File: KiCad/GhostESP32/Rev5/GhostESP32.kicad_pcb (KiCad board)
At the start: 2 copper layers, 76.7 x 56.7 mm, 52 parts, among them J1 USB_OTG, J2 CONN_01X12, J3 CONN_01X12, J4 STEERING, J5 MOTOR, Q1 Q_NPN_BEC, Q2 Q_NPN_BEC, Q3 Q_NPN_BEC, Q4 BSS138, Q5 BSS138, SW1 SW_SPDT, U1 NCP1117-3.3_SOT223, U2 CP2102, U3 TMP102, U4 MPU-9250, U5 ESP-WROOM-32, U6 NeoPixelNano, U7 NeoPixelNano

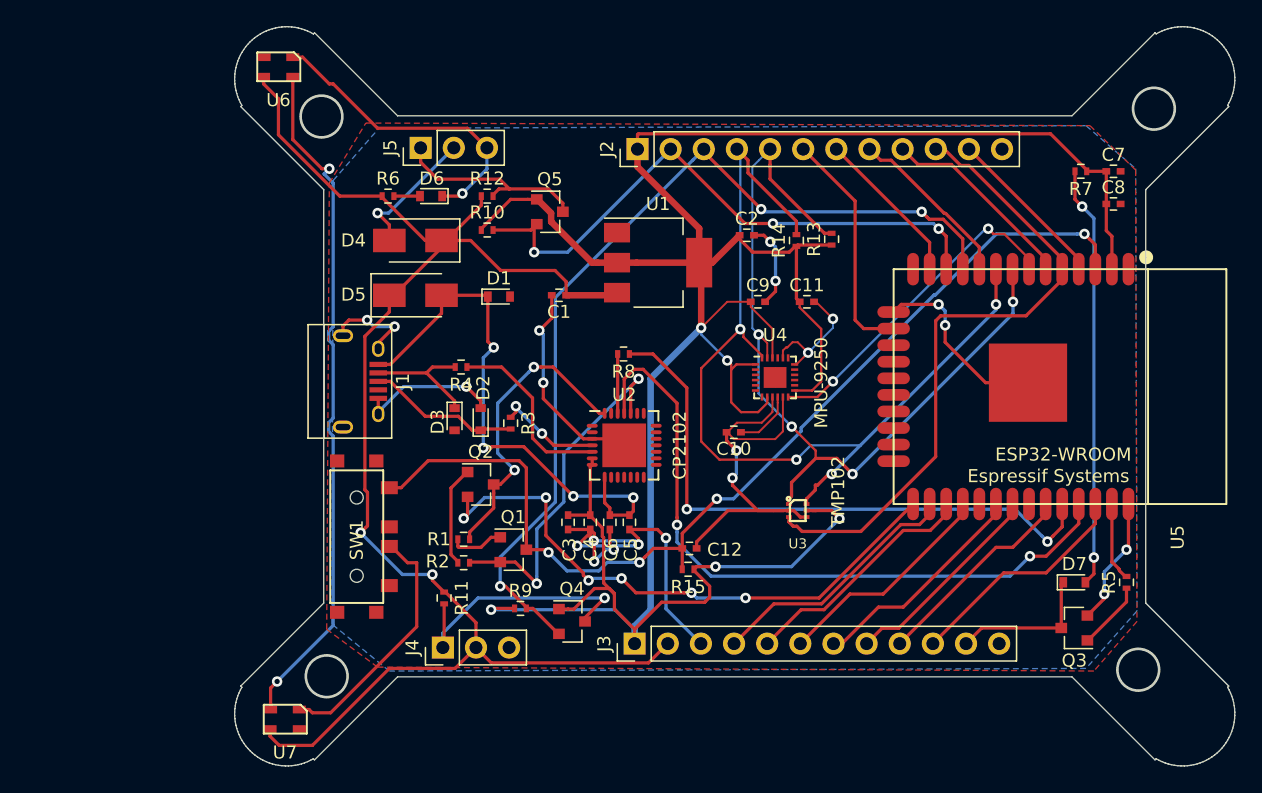
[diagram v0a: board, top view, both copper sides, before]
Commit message: Working on revision 5 of the PCBs
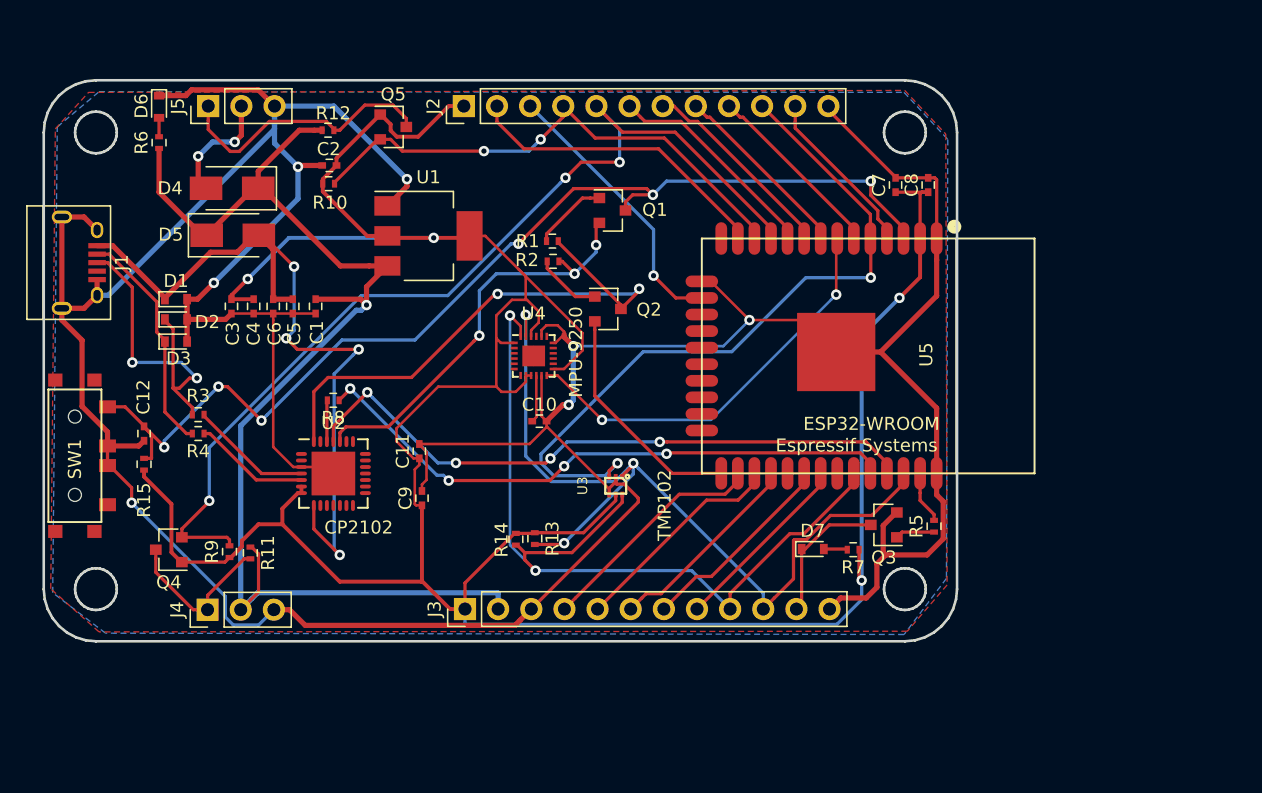
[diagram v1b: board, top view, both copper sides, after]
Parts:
- removed U6, U7: NeoPixelNano, NorBotKiCadFootprints:NeoPixelNano
- R13, R14: value 2k2 -> 10k
- moved C12 42.7 mm to (102.7, 108.6), turned to 270 degrees
- moved R15 42.5 mm to (102.7, 111.0), turned to 90 degrees
- moved R7 33.8 mm to (157.1, 117.5)
- moved C2 32.4 mm to (116.9, 88.0), turned to 180 degrees
- moved R13 32.3 mm to (132.7, 116.7), turned to 270 degrees
- moved C11 31.8 mm to (123.8, 110.0), turned to 90 degrees
- moved R14 31.4 mm to (131.2, 116.7), turned to 270 degrees
- moved Q4 31.4 mm to (104.6, 117.5), turned to 180 degrees
- moved C4 30.7 mm to (111.1, 98.8)
- moved C5 30.7 mm to (114.1, 98.8)
- moved C6 30.7 mm to (112.6, 98.8)
- moved C3 30.7 mm to (109.4, 98.8)
- moved C9 29.8 mm to (124.0, 113.5), turned to 90 degrees
- moved Q1 27.1 mm to (138.6, 91.5)
- moved D1 24.8 mm to (105.2, 98.3)
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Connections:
- J2 pad 2: IO27 -> IO14
- J2 pad 3: IO26 -> IO13
- J2 pad 4: IO33/SDA -> IO27
- J2 pad 5: IO32/SCL -> IO26
- J2 pad 6: IO13 -> IO25
- J2 pad 7: IO14 -> IO33
- J2 pad 8: IO25 -> IO32
- J3 pad 10: IO22 -> IO22(SCL)
- J3 pad 9: IO21 -> IO21(SDA)
- R13 pad 2: IO32/SCL -> IO22(SCL)
- R14 pad 2: IO33/SDA -> IO21(SDA)
- U3 pad 1: IO32/SCL -> IO22(SCL)
- U3 pad 6: IO33/SDA -> IO21(SDA)
- U4 pad 23: IO32/SCL -> IO22(SCL)
- U4 pad 24: IO33/SDA -> IO21(SDA)
- U4 pad 9: GND -> +3V3
- U5 pad 33: IO21 -> IO21(SDA)
- U5 pad 36: IO22 -> IO22(SCL)
- U5 pad 8: IO32/SCL -> IO32
- U5 pad 9: IO33/SDA -> IO33
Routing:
- net GND: track 181.8 -> 313.2 mm, vias 22 -> 7
- net IO33/SDA: track 72.6 -> 0.00 mm, vias 4 -> 0
- net IO22(SCL): track 0.00 -> 66.7 mm, vias 0 -> 3
- net IO21(SDA): track 0.00 -> 65.7 mm, vias 0 -> 2
- net IO32/SCL: track 65.6 -> 0.00 mm, vias 4 -> 0
- net Net-(U6-Pad1): track 53.0 -> 0.00 mm, vias 2 -> 0
- net Net-(D7-Pad2): track 32.4 -> 1.82 mm, vias 2 -> 0
- net IO0: track 45.0 -> 17.9 mm, vias 6 -> 0
- net +5V: track 116.7 -> 96.2 mm, vias 2 -> 1
- net DTR: track 23.5 -> 41.3 mm
- net IO22: track 17.8 -> 0.00 mm
- net VBUS: track 42.8 -> 59.7 mm
- net IO21: track 16.1 -> 0.00 mm
- net IO33: track 0.00 -> 15.5 mm
- net IO32: track 0.00 -> 14.2 mm
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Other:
- board size 76.7 x 56.7 mm -> 70 x 43 mm
- net class 3V3 added: clearance 0.2, trace_width 0.3, via_dia 0.8, via_drill 0.4
- net class 5V added: clearance 0.2, trace_width 0.4, via_dia 0.8, via_drill 0.4
- net class GND added: clearance 0.2, trace_width 0.4, via_dia 0.8, via_drill 0.4
- net class Thin added: clearance 0.2, trace_width 0.2, via_dia 0.8, via_drill 0.4
- board text added: "Ghost32 Rev 5 Frode Lillerud 17.mar 2018"
- board text added: "IO21(SDA)"
- board text added: "IO22(SCL)"
- board text added: "IO32"
- board text added: "IO33"
- board text removed: "Ghost32 Rev 5 Frode Lillerud 9.feb 2018"
- board text removed: "IO21"
- board text removed: "IO22"
- board text removed: "SCL/IO32"
- board text removed: "SDA/IO33"
